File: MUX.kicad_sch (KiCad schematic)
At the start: 24 parts, among them U15 CD74HC4067SM, U21 CD74HC4067SM, U51 CD74HC4067SM, U56 CD74HC4067SM, U62 CD74HC4067SM, U68 CD74HC4067SM, U69 CD74HC4067SM, U74 CD74HC4067SM

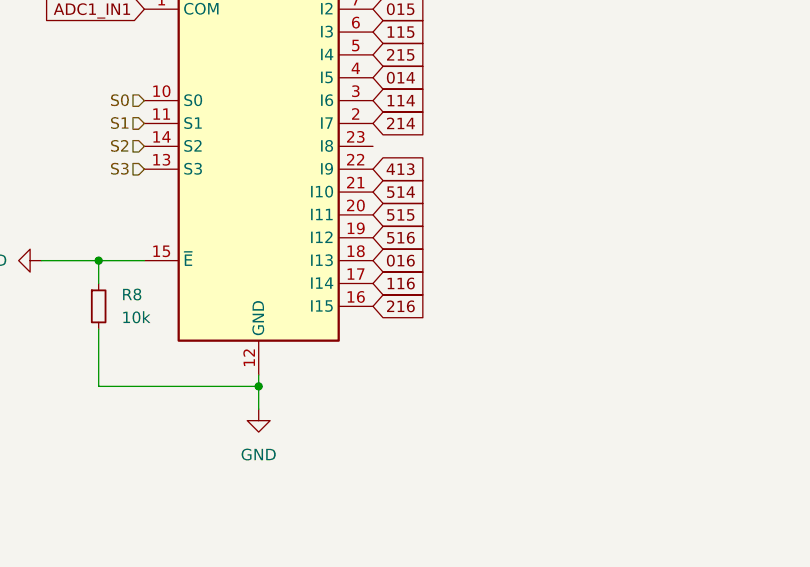
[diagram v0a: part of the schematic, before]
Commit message: Final trace
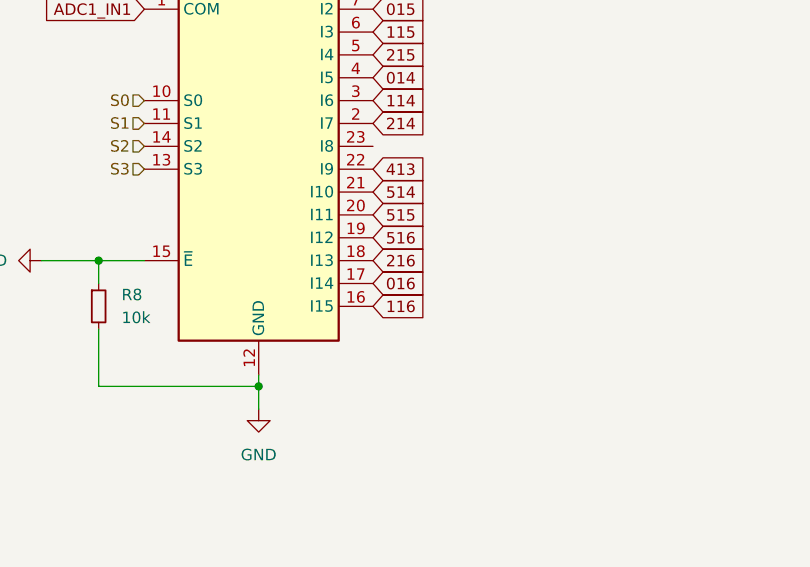
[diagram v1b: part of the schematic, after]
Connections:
- net 016: now also U74.17 (I14); no longer U74.18 (I13)
- net 116: now also U74.16 (I15); no longer U74.17 (I14)
- net 216: now also U74.18 (I13); no longer U74.16 (I15)
